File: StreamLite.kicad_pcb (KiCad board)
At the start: 2 copper layers, 78.5 x 48.5 mm, 60 parts, among them J2 Screw_Terminal_01x03, J3 Conn_01x06_Socket, J4 Screw_Terminal_01x03, J5 Screw_Terminal_01x03, J6 Screw_Terminal_01x03, J7 Screw_Terminal_01x03, J8 Screw_Terminal_01x03, Q1 BC327, Q10 BC327, Q11 BC337, Q13 AO3400A, Q2 BC337, Q3 AO3400A, Q4 BC327, Q5 BC337, Q6 AO3400A, Q7 BC327, Q8 BC337, Q9 AO3400A, SW1 Reset, U2 ESP32-WROOM-32, U3 AMS1117-3.3

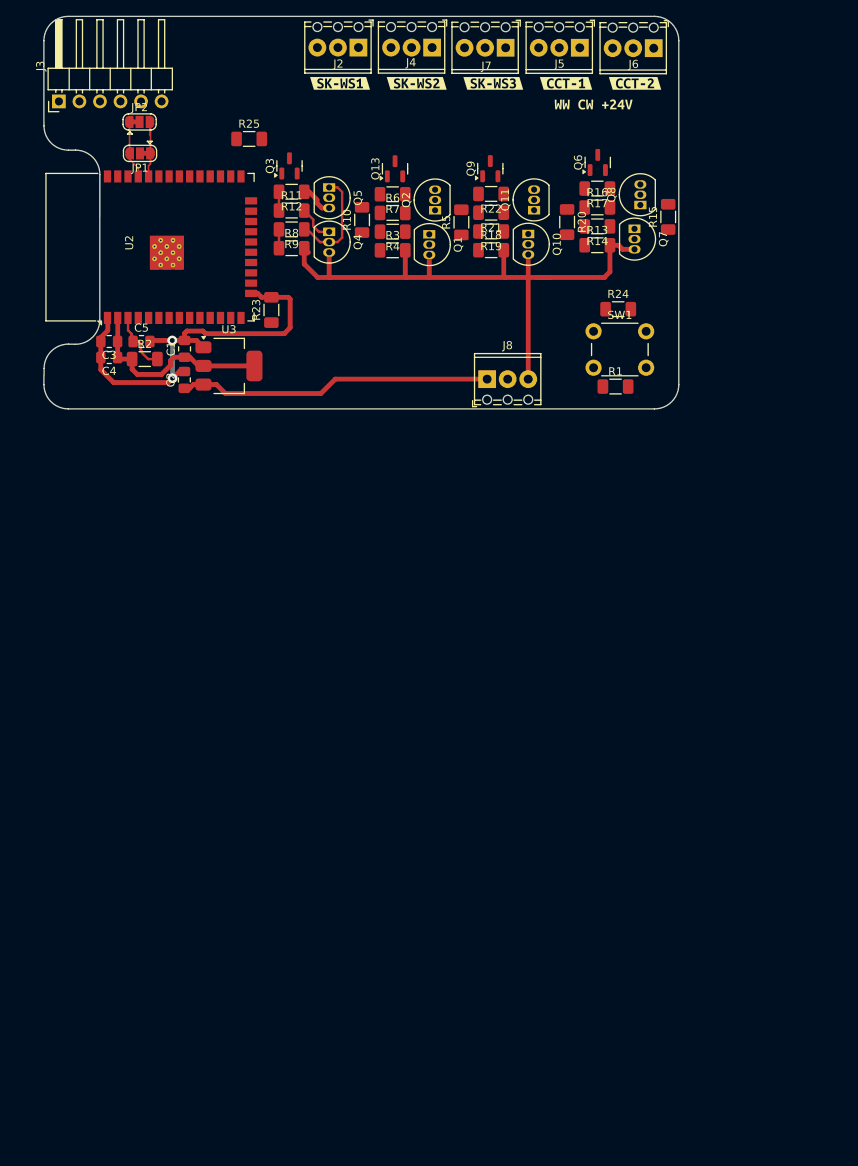
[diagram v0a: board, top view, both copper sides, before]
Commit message: add more parts
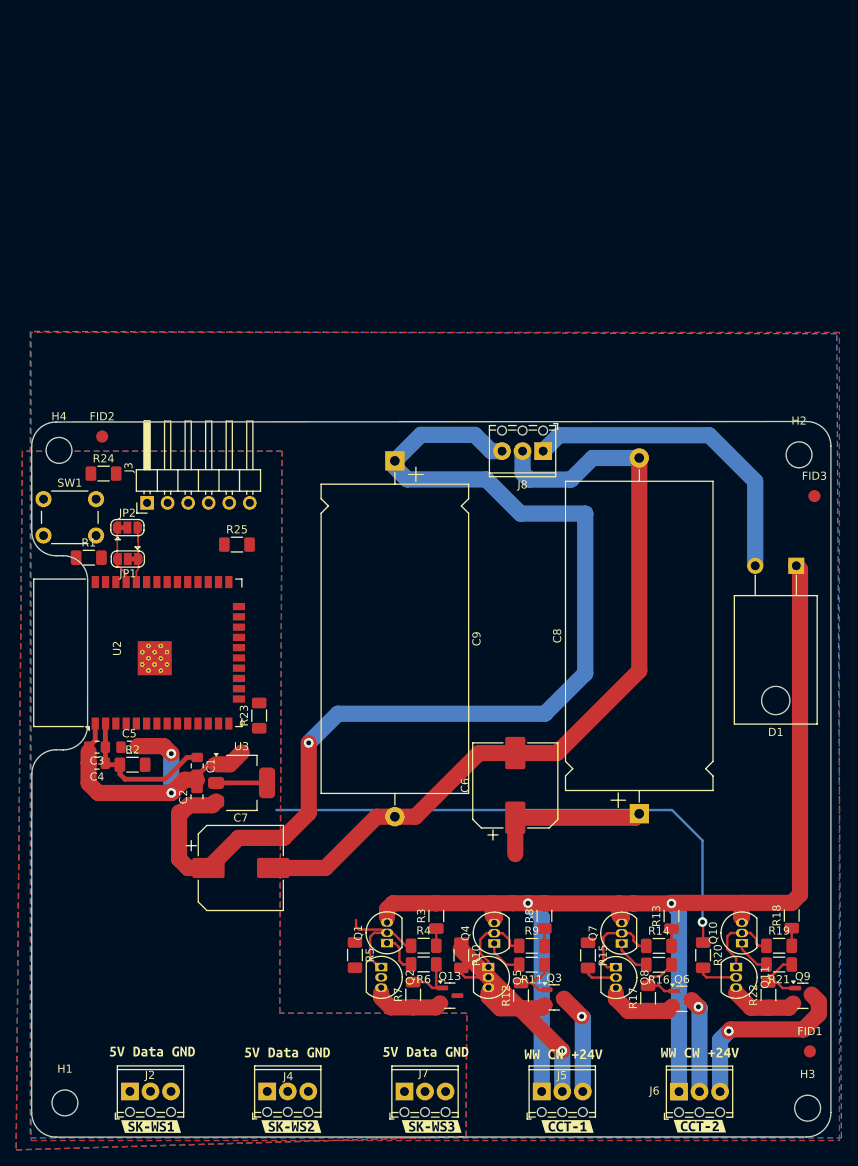
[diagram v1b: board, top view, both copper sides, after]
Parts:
- added C6: 470u, Capacitor_SMD:CP_Elec_10x10, F.Cu at (99.2, 135.9)
- added C7: 470u, Capacitor_SMD:CP_Elec_10x10, F.Cu at (65.2, 146.1)
- added C8: 10.000uF, Capacitor_THT:CP_Axial_L38.0mm_D18.0mm_P44.00mm_Horizontal, F.Cu at (114.5, 139.4)
- added C9: 10.000uF, Capacitor_THT:CP_Axial_L38.0mm_D18.0mm_P44.00mm_Horizontal, F.Cu at (84.3, 95.8)
- added D1: D, Package_TO_SOT_THT:TO-220-2_Horizontal_TabDown, F.Cu at (133.9, 108.7)
- added FID1: Fiducial, Fiducial:Fiducial_1.5mm_Mask3mm, F.Cu at (135.6, 168.8)
- added FID2: Fiducial, Fiducial:Fiducial_1.5mm_Mask3mm, F.Cu at (48.1, 92.8)
- added FID3: Fiducial, Fiducial:Fiducial_1.5mm_Mask3mm, F.Cu at (136.2, 100.1)
- added H1: MountingHole, MountingHole:MountingHole_3.2mm_M3, F.Cu at (43.5, 175.2)
- added H2: MountingHole, MountingHole:MountingHole_3.2mm_M3, F.Cu at (134.2, 95.0)
- added H3: MountingHole, MountingHole:MountingHole_3.2mm_M3, F.Cu at (135.3, 175.8)
- added H4: MountingHole, MountingHole:MountingHole_3.2mm_M3, F.Cu at (42.7, 94.5)
- added kibuzzard-670D99B4: G***, kibuzzard-670D99B4, F.Cu at (105.1, 169.1)
- added kibuzzard-670EF22D: G***, kibuzzard-670EF22D, F.Cu at (88.1, 168.8)
- added kibuzzard-670EF237: G***, kibuzzard-670EF237, F.Cu at (71.0, 168.9)
- added kibuzzard-670EF243: G***, kibuzzard-670EF243, F.Cu at (54.3, 168.8)
- moved J2 132.1 mm to (51.5, 173.7), turned to 0 degrees
- moved kibuzzard-670D983B 131.1 mm to (54.1, 178.1)
- moved J4 130.7 mm to (68.5, 173.7), turned to 0 degrees
- moved kibuzzard-670D9849 129.9 mm to (71.5, 178.1)
- moved J7 129.7 mm to (85.5, 173.7), turned to 0 degrees
- moved kibuzzard-670D9857 129.2 mm to (88.8, 178.1)
- moved kibuzzard-670D97D1 129.2 mm to (122.0, 178.0)
- moved J5 129.2 mm to (102.4, 173.7), turned to 0 degrees
- moved J6 129.1 mm to (119.4, 173.8), turned to 0 degrees
- moved kibuzzard-670D998F 129.0 mm to (105.6, 178.1)
- moved kibuzzard-670D99B4 118.0 mm to (122.0, 168.9)
- moved Q9 109.3 mm to (134.7, 161.9), turned to 0 degrees
- moved Q3 107.9 mm to (104.0, 162.1), turned to 0 degrees
- moved R22 104.8 mm to (130.5, 161.8), turned to 90 degrees
- moved Q6 103.9 mm to (119.8, 162.3), turned to 0 degrees
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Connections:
- J2 pad 1: +3V3 -> +5V
- J4 pad 1: +3V3 -> +5V
- J7 pad 1: +3V3 -> +5V
- J8 pad 1: +5V -> /V_IN
- J8 pad 3: +24V -> +5V
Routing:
- net GND: track 57.4 -> 173.0 mm
- net +5V: track 38.8 -> 146.7 mm, vias 0 -> 1
- net +24V: track 77.9 -> 167.1 mm, vias 0 -> 2
- net CCT1_WW: track 0.00 -> 66.9 mm, vias 0 -> 1
- net /V_IN: track 0.00 -> 39.8 mm
- net /CW1: track 0.00 -> 22.8 mm, vias 0 -> 1
- net /WW2: track 0.00 -> 22.7 mm, vias 0 -> 1
- net Net-(Q1-B): track 0.00 -> 14.6 mm
- net /WW1: track 0.00 -> 12.5 mm, vias 0 -> 1
- net /CW2: track 0.00 -> 11.7 mm, vias 0 -> 1
- net Net-(Q7-B): track 0.00 -> 11.5 mm
- net Net-(Q10-B): track 0.00 -> 10.3 mm
- net Net-(Q6-G): track 0.00 -> 7.94 mm
- net Net-(Q9-G): track 0.00 -> 7.83 mm
- net Net-(U2-EN): track 7.66 -> 0.00 mm
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- added copper zone on F.Cu, net +24V
- added copper zone on B.Cu, net GND
- added copper zone on F.Cu, net GND
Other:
- board size 78.5 x 48.5 mm -> 98.8 x 88.5 mm
